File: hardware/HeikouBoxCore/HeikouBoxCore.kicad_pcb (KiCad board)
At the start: 2 copper layers, 40 x 40 mm, 28 parts, among them U1 EP3C25E144

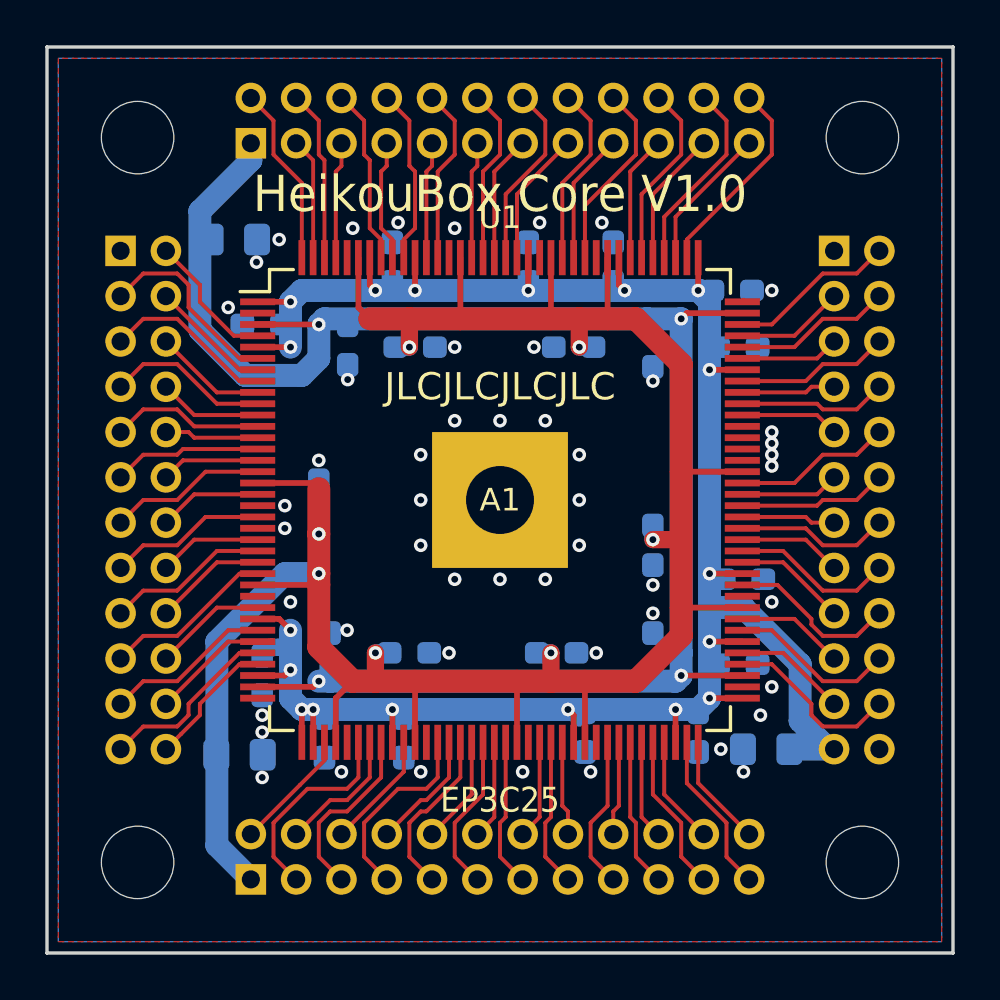
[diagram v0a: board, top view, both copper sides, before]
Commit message: Okay let's do this properly
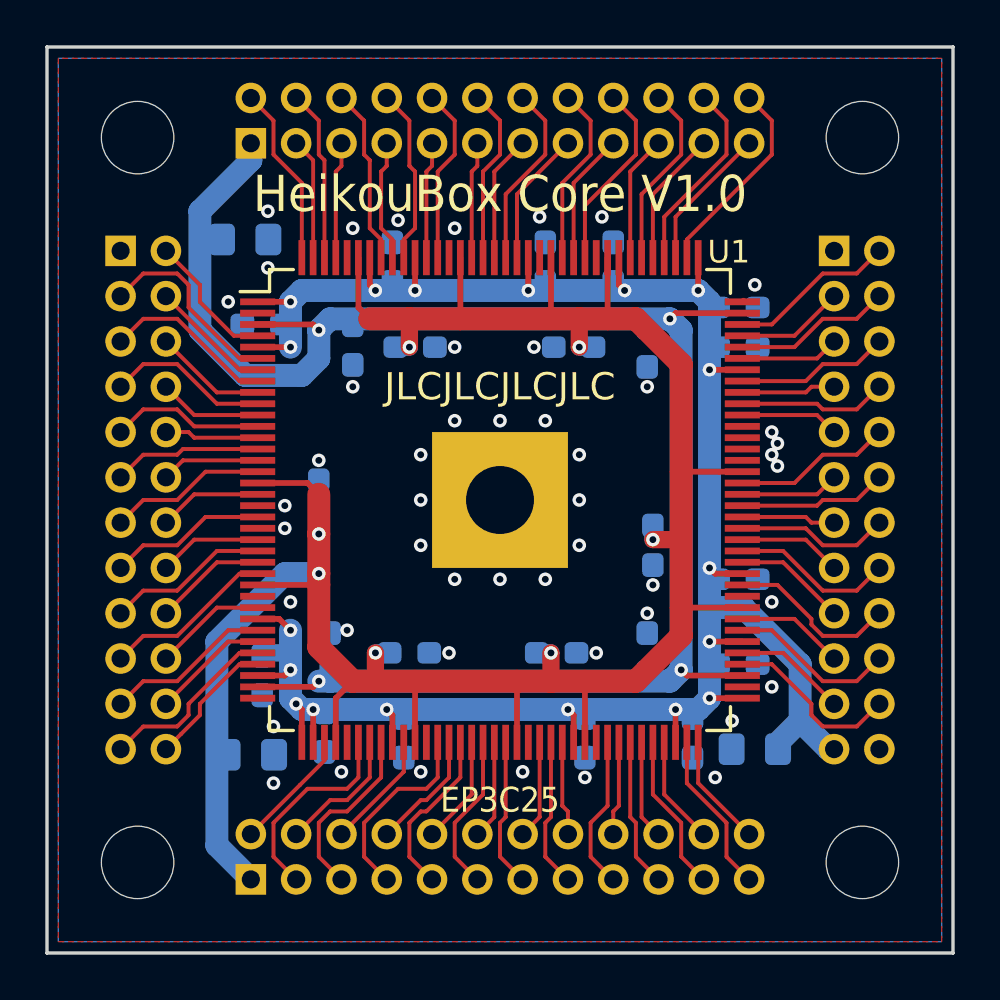
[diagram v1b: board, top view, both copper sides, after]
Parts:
- removed A1: HeikouBox-Core, ksk-heikoubox:HeikouBox-Core-Top
- added J1: L, KSK_HeikouBox:PinHeader_2x12_P2.00mm_Vertical-MIRRORED, B.Cu at (22.2, 26.0)
- added J2: B, KSK_HeikouBox:PinHeader_2x12_P2.00mm_Vertical-MIRRORED, B.Cu at (26.0, 51.8)
- added J3: R, KSK_HeikouBox:PinHeader_2x12_P2.00mm_Vertical-MIRRORED, B.Cu at (53.8, 26.0)
- added J4: T, KSK_HeikouBox:PinHeader_2x12_P2.00mm_Vertical-MIRRORED, B.Cu at (26.0, 19.2)
- added MH1: M3, MountingHole:MountingHole_3.2mm_M3, F.Cu at (21.0, 21.0)
- added MH2: M3, MountingHole:MountingHole_3.2mm_M3, F.Cu at (53.0, 21.0)
- added MH3: M3, MountingHole:MountingHole_3.2mm_M3, F.Cu at (21.0, 53.0)
- added MH4: M3, MountingHole:MountingHole_3.2mm_M3, F.Cu at (53.0, 53.0)
- U1: footprint ksk-heikoubox:EQFP-144-HANDSOLDER -> KSK_HeikouBox:EQFP-144-HANDSOLDER
- moved C11 0.79 mm to (47.5, 28.5)
- moved C9 0.75 mm to (39.0, 26.5)
- moved C24 0.50 mm to (26.0, 48.2)
- moved C25 0.50 mm to (25.8, 25.5)
- moved C26 0.50 mm to (48.2, 48.0)
- moved C15 0.35 mm to (45.5, 47.5)
- moved C13 0.25 mm to (47.5, 40.5)
- moved C16 0.25 mm to (40.8, 47.5)
- moved C18 0.25 mm to (29.2, 47.2)
- moved C21 0.25 mm to (43.5, 30.2)
- moved C22 0.25 mm to (43.5, 43.8)
- moved C20 0.22 mm to (30.5, 30.2)
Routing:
- net /V12: track 106.1 -> 100.4 mm
- net /V25: track 76.5 -> 77.5 mm
- net /GND: vias 50 -> 48
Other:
- net class Power added: clearance 0.175, trace_width 0.508, via_dia 0.8, via_drill 0.4
- net class PowerSub added: clearance 0.175, trace_width 0.254, via_dia 0.8, via_drill 0.4
- net class Signal added: clearance 0.175, trace_width 0.1524, via_dia 0.8, via_drill 0.4
